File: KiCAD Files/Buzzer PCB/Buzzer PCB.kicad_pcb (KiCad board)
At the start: 2 copper layers, 25.2 x 22.9 mm, 14 parts, among them J1 JST-PH Battery IN, J2 JST-PH Feather BAT OUT, J3 Comidox Boost Module, J4 Feather D13, Q1 S8050, SW1 SS12D00G5

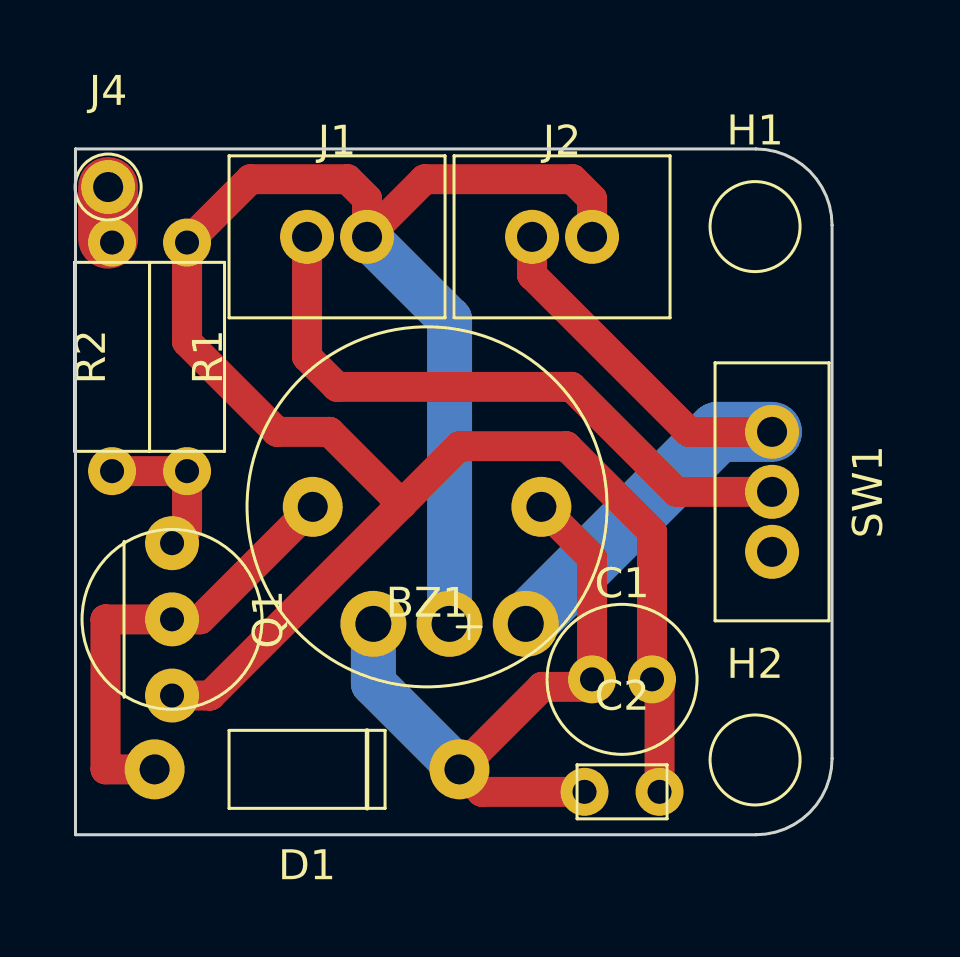
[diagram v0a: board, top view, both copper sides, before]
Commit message: FlatCAM ready
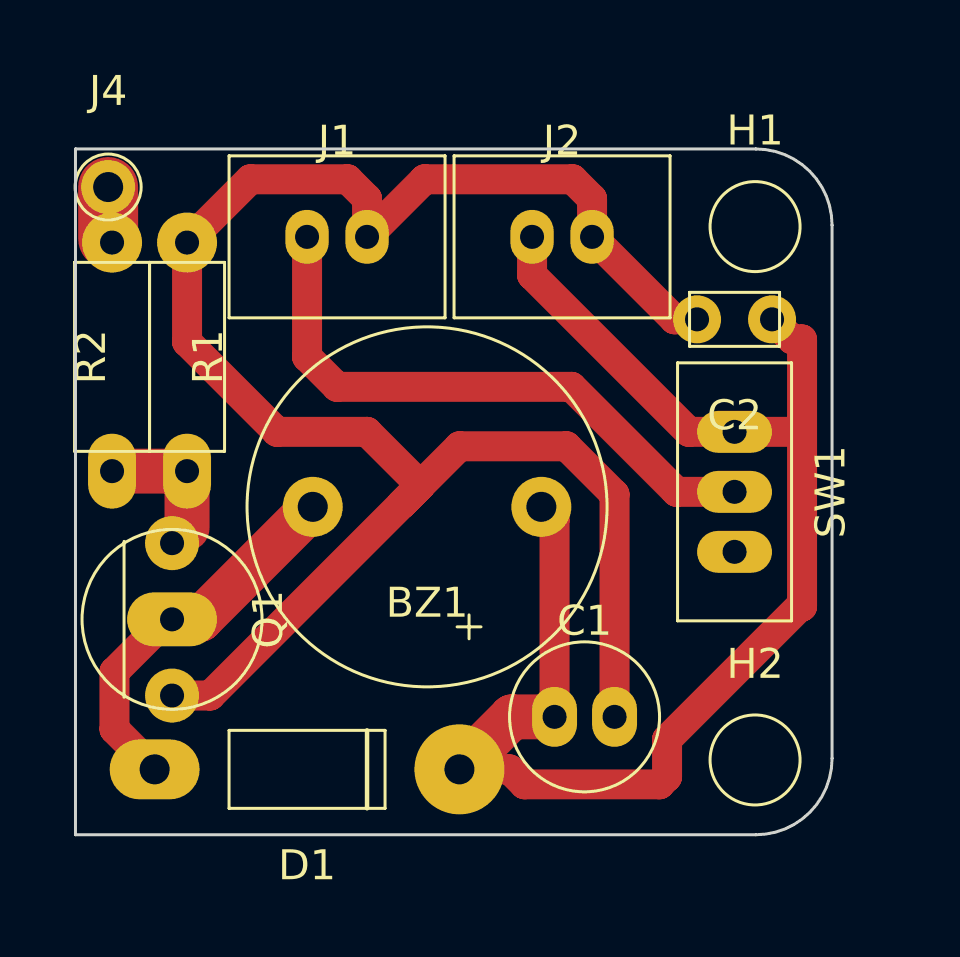
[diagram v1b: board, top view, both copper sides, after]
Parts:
- removed J3: Comidox Boost Module, Module:Comidox_Boost_11x11_3Pin_Custom
- moved C2 16.2 mm to (106.8, 97.2), turned to 180 degrees
- moved C1 1.77 mm to (101.8, 110.5)
- moved SW1 1.25 mm to (106.8, 103.0)
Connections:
- BZ1 pad 1: BOOST_5V -> SW_BAT
- C1 pad 1: BOOST_5V -> SW_BAT
- C2 pad 1: BOOST_5V -> SW_BAT
- D1 pad 1: BOOST_5V -> SW_BAT
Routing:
- net SW_BAT: track 22.3 -> 48.5 mm
- net BOOST_5V: track 22.5 -> 0.00 mm
- net GND: track 74.4 -> 63.1 mm
- net BUZZER_LOW: track 15.1 -> 12.7 mm
- net BAT_IN: track 21.4 -> 20.1 mm
